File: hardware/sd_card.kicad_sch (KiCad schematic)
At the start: 2 parts

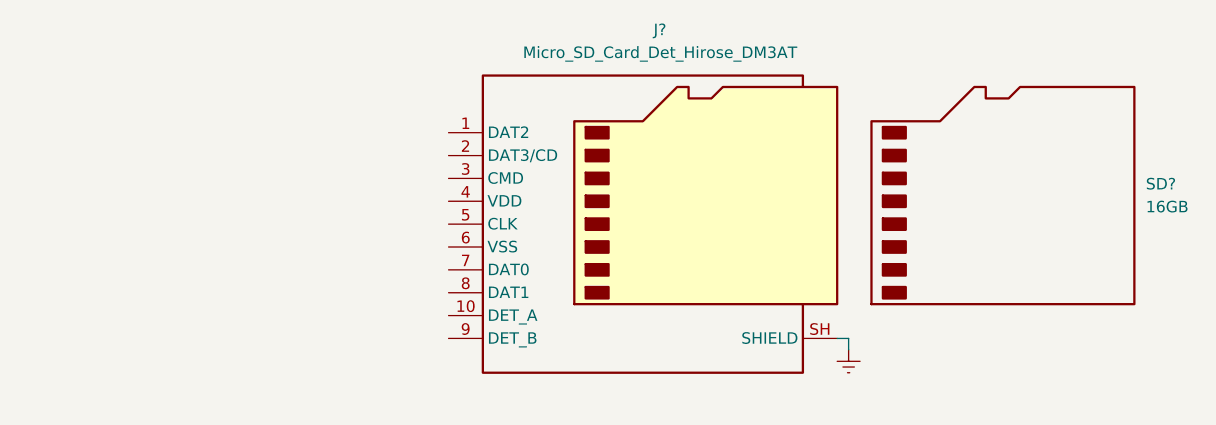
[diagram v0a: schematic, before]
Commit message: Random changes & LED additions
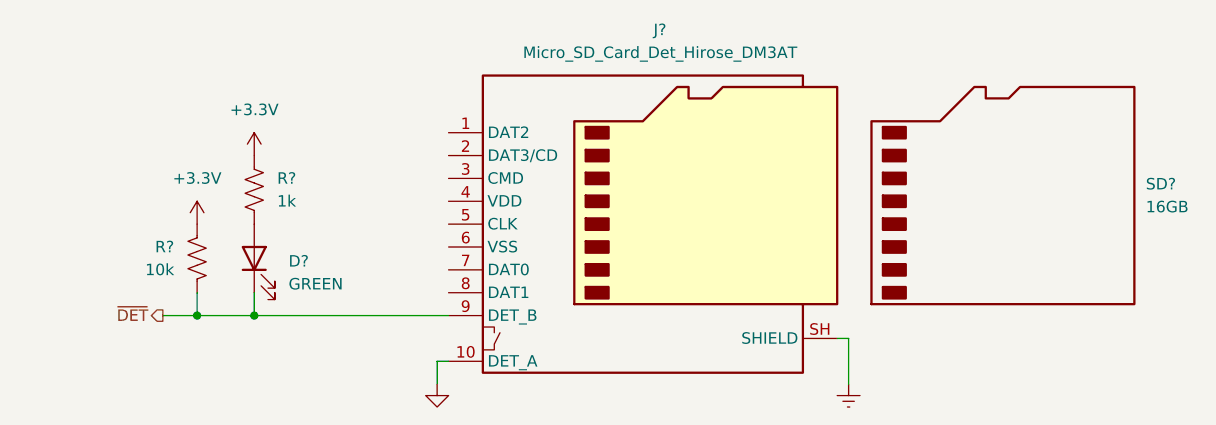
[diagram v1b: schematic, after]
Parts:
- added D?: GREEN, Diode_SMD:D_0805_2012Metric, symbol Device:LED
- added R?: 10k, Resistor_SMD:R_0603_1608Metric, symbol Device:R_US
- added R?: 1k, Resistor_SMD:R_0603_1608Metric, symbol Device:R_US
- J?: Part Number (none) -> DM3AT-SF-PEJM5; Vendor URL (none) -> https://www.digikey.com/en/products/detail/hirose-electric-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
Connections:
- net GND: now reaches J?.10 (DET_A)
- net ~{DET}: now reaches J?.9 (DET_B)
- net ~{DET}: now also D?.1 (K), R?.2
- new net: D?.2 (A), R?.2
- new net +3.3V: R?.1, R?.1

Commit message: Connector Updates
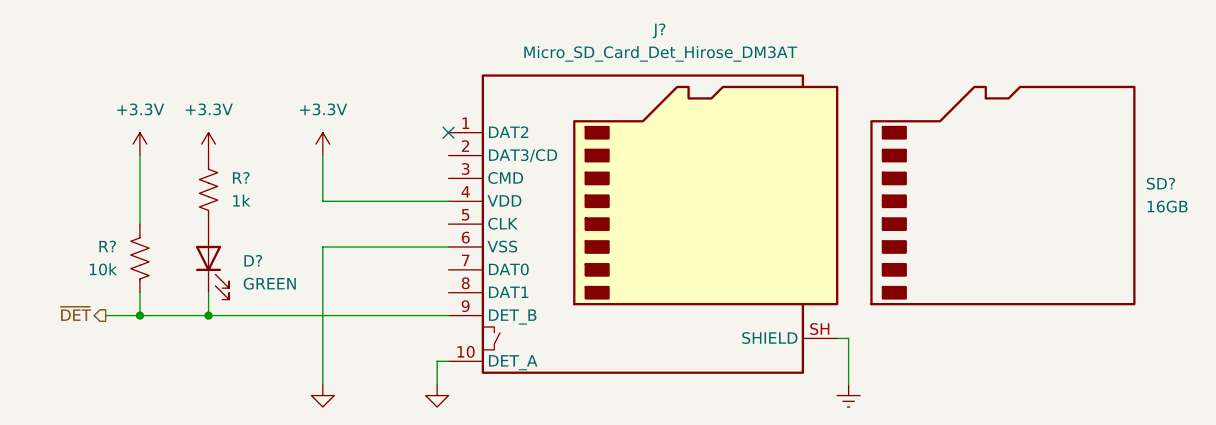
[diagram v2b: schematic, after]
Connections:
- net +3.3V: now also J?.4 (VDD)
- net GND: now also J?.6 (VSS)
- no-connect marks 0 -> 1
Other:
- moved on the sheet: D?, R?
